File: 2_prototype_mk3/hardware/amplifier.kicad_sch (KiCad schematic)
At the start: 8 parts, among them U5 MAX98357A

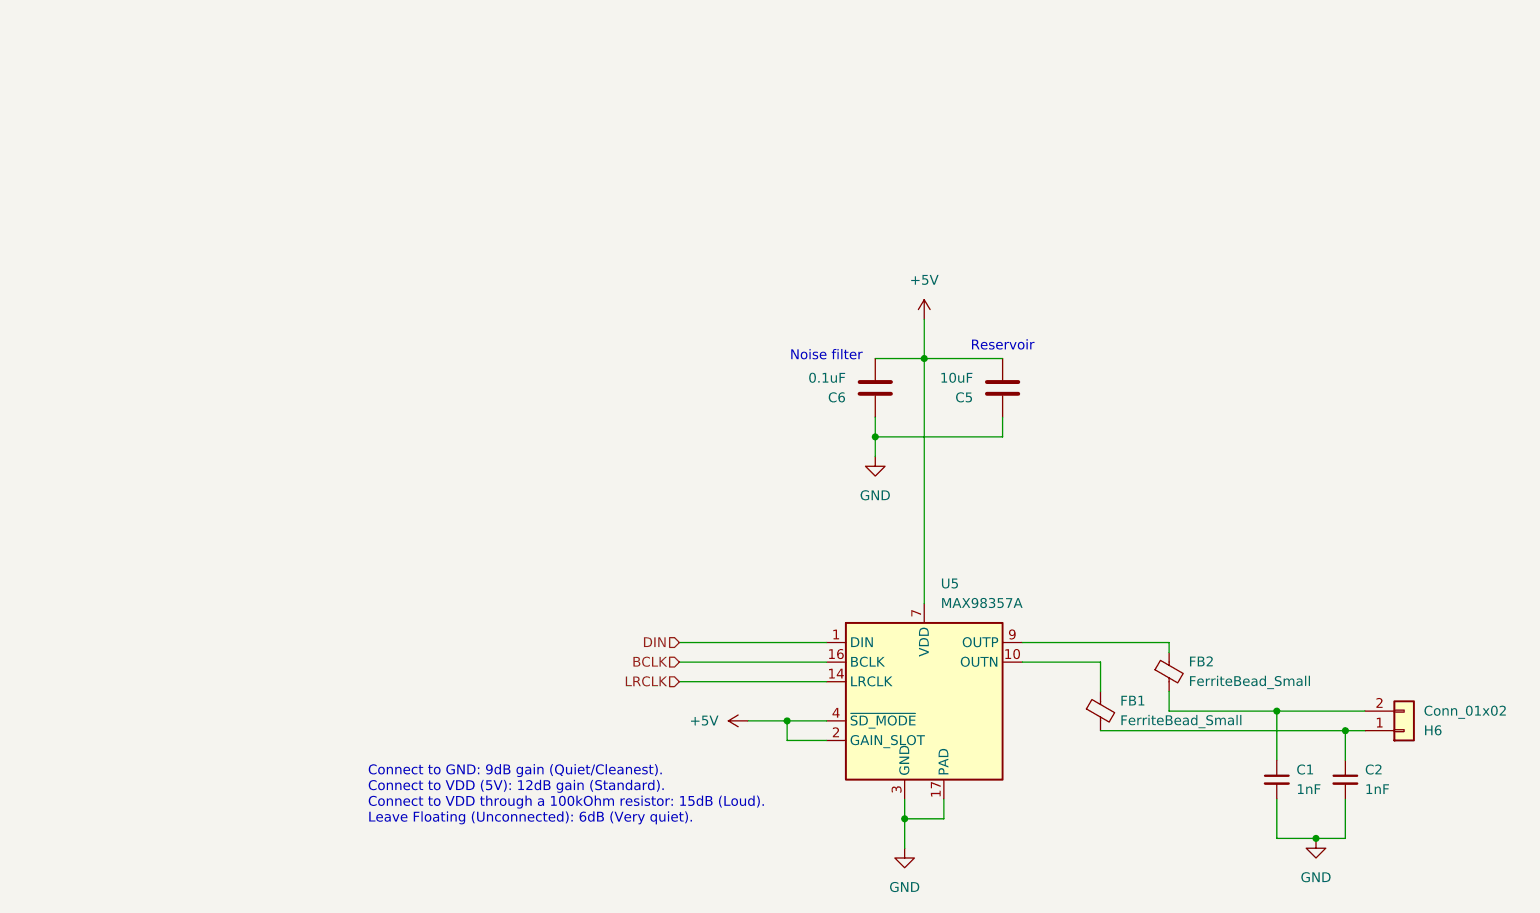
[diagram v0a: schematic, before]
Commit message: MKIII design refinements
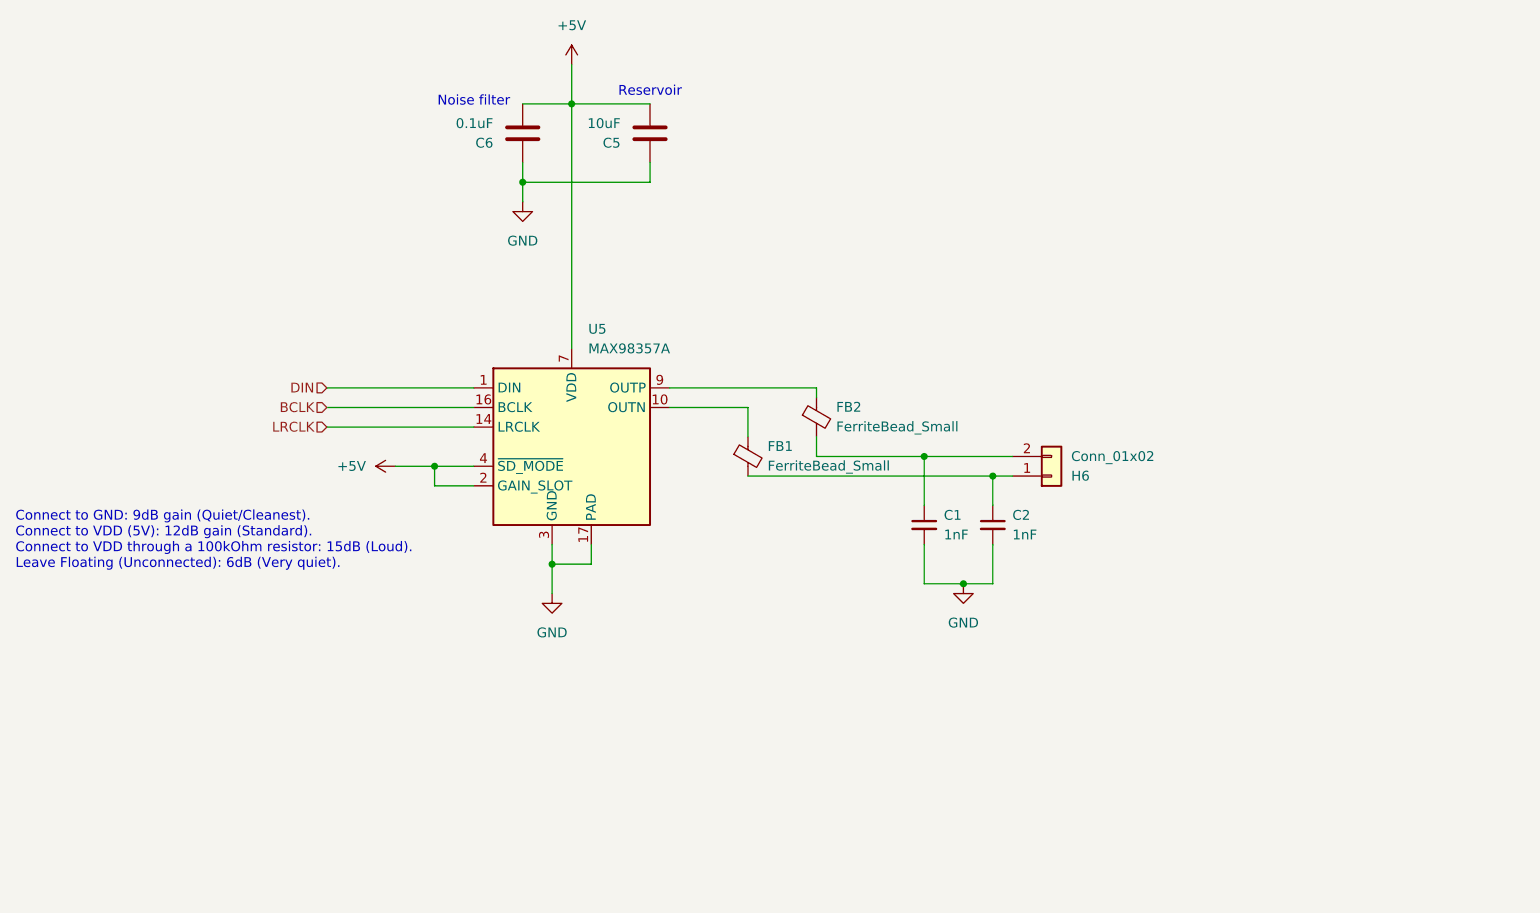
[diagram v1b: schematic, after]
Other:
- title: (none) -> Amplifier
- moved on the sheet: C1, C2, C5, C6, FB1, FB2, H6, U5
